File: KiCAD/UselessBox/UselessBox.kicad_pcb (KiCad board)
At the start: 2 copper layers, 13 parts, among them J1 Power IN, J2 Switch (2 x On), J4 Servo Door, J5 Servo Finger, J6 Calibration Switches, K1 G5V-2, Q1 BC107

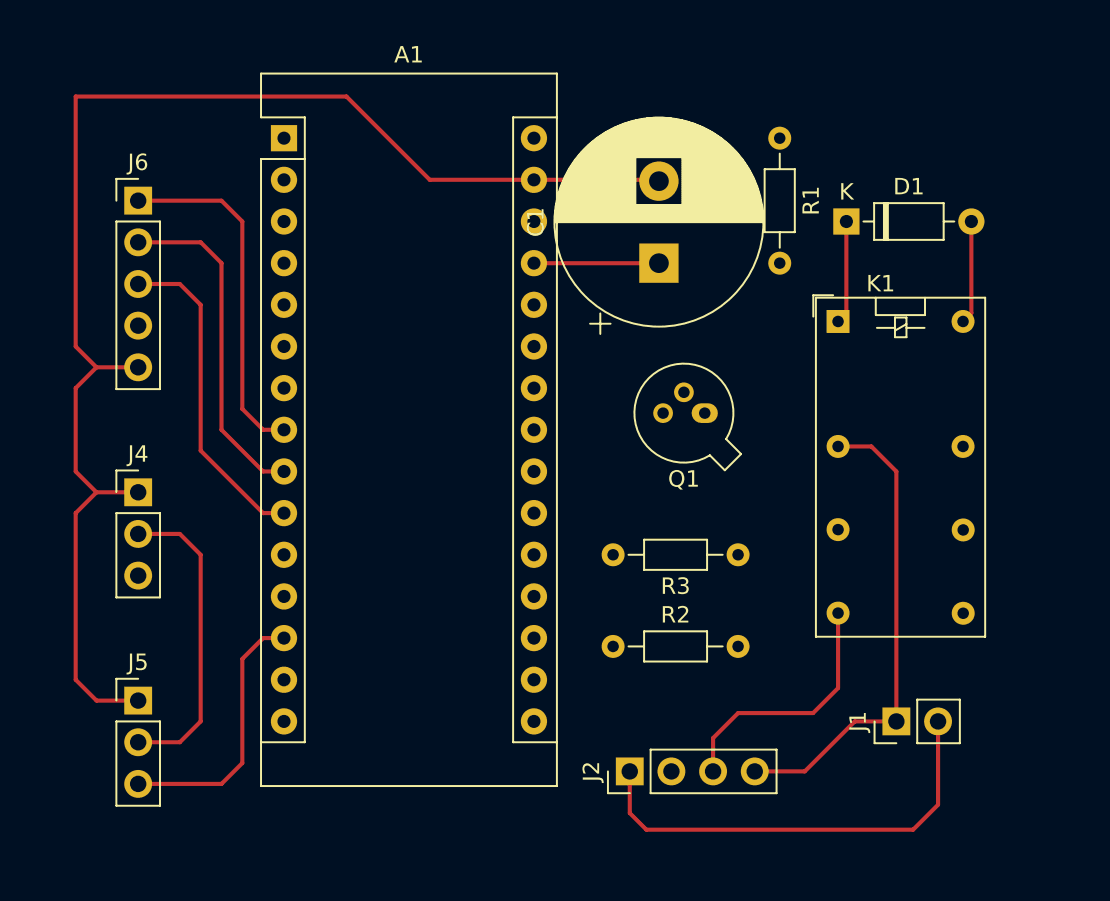
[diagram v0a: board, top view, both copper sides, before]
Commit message: PCB completed
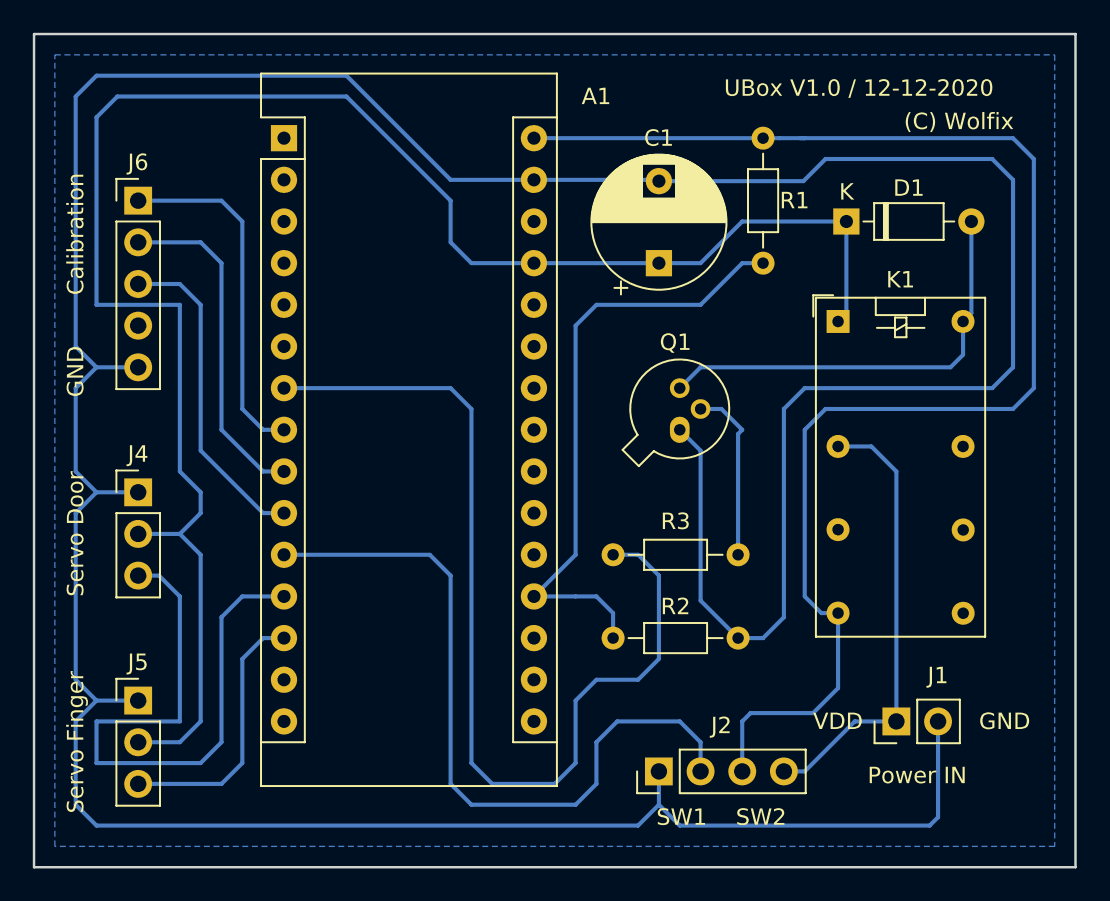
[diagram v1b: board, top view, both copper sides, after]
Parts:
- C1: footprint Capacitor_THT:CP_Radial_D12.5mm_P5.00mm -> Capacitor_THT:CP_Radial_D8.0mm_P5.00mm
- moved Q1 1.83 mm to (119.4, 99.1), turned to 90 degrees
- moved J2 1.78 mm to (118.1, 119.9)
- moved R1 1.02 mm to (124.5, 81.3)
- moved R2 0.51 mm to (115.3, 111.8)
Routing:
- net Net-(A1-Pad29): track 112.2 -> 234.3 mm
- net Net-(A1-Pad27): track 32.8 -> 109.7 mm
- net Net-(A1-Pad30): track 15.5 -> 87.2 mm
- net Net-(A1-Pad7): track 0.00 -> 59.3 mm
- net Net-(A1-Pad11): track 0.00 -> 45.0 mm
- net Net-(A1-Pad12): track 0.00 -> 38.4 mm
- net Net-(A1-Pad19): track 0.00 -> 37.3 mm
- net Net-(D1-Pad2): track 6.31 -> 26.5 mm
- net Net-(Q1-Pad2): track 0.00 -> 10.8 mm
- net Net-(J1-Pad1): track 29.3 -> 27.5 mm
- added copper zone on B.Cu, net Net-(A1-Pad29)
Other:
- board outline added: 63.5 x 50.8 mm
- rule pad_to_mask_clearance: 0.051 -> 0
- board text added: "(C) Wolfix"
- board text added: "Calibration"
- board text added: "GND"
- board text added: "Power IN"
- board text added: "SW1 SW2"
- board text added: "Servo Door"
- board text added: "Servo Finger"
- board text added: "UBox V1.0 / 12-12-2020"
- board text added: "VDD"
